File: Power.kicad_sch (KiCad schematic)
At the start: 41 parts, among them Q1 DMP2065UFDB, U6 TPS62180, U7 CYPD3177-24LQ, U8 TPS82130, U9 DS1307Z+, Y1 32.768kHz

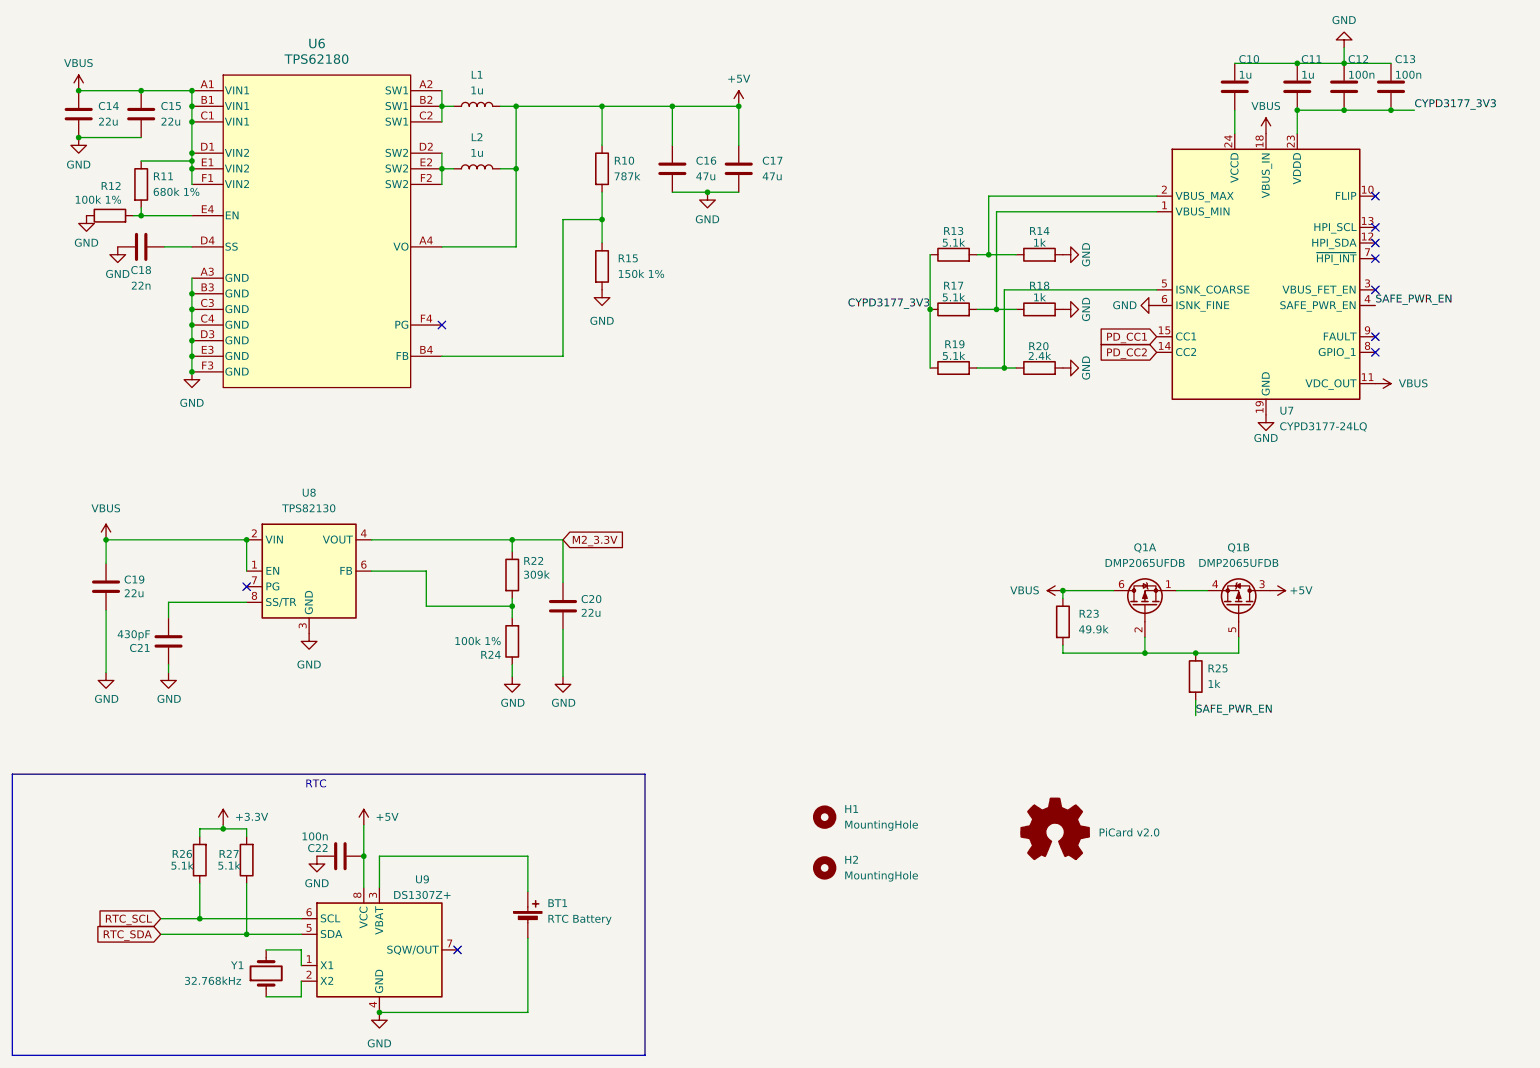
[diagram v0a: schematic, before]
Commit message: Update
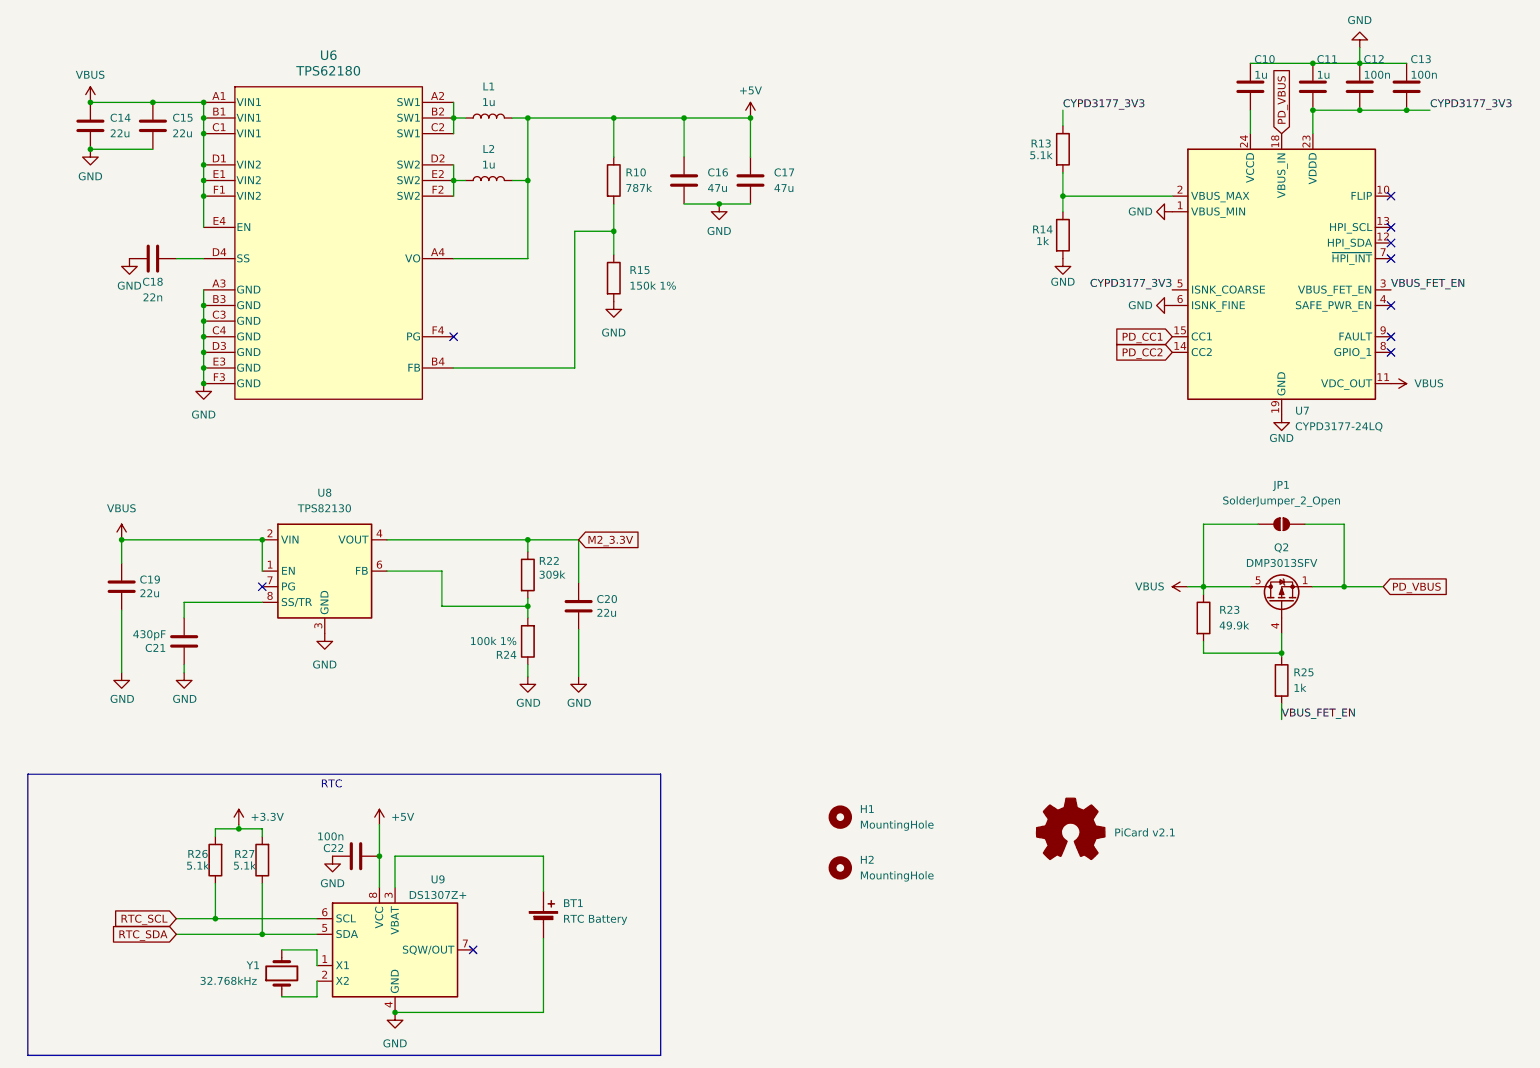
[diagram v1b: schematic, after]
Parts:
- removed Q1: DMP2065UFDB, PiCard:DFN200X200X60-8N, symbol Device:Q_Dual_PMOS_S1G1D2S2G2D1
- removed R11: 680k 1%, Resistor_SMD:R_0402_1005Metric, symbol Device:R
- removed R12: 100k 1%, Resistor_SMD:R_0402_1005Metric, symbol Device:R
- removed R17, R19: 5.1k, Resistor_SMD:R_0402_1005Metric, symbol Device:R
- removed R18: 1k, Resistor_SMD:R_0402_1005Metric, symbol Device:R
- removed R20: 2.4k, Resistor_SMD:R_0402_1005Metric, symbol Device:R
- added JP1: SolderJumper_2_Open, Jumper:SolderJumper-2_P1.3mm_Open_TrianglePad1.0x1.5mm, symbol Jumper:SolderJumper_2_Open
- added Q2: DMP3013SFV, Package_SON:Diodes_PowerDI3333-8, symbol Transistor_FET:DMP3013SFV
- SYM1: value PiCard v2.0 -> PiCard v2.1
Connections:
- net CYPD3177_3V3: now also U7.5 (ISNK_COARSE)
- net GND: now also U7.1 (VBUS_MIN)
- net VBUS: now also U6.E4 (EN), JP1.1 (A), Q2.5 (D); no longer U7.18 (VBUS_IN)
- net at R23.2, R25.1: now also Q2.4 (G)
- net VBUS_FET_EN: now reaches U7.3 (VBUS_FET_EN)
- net VBUS_FET_EN: now also R25.2
- net SAFE_PWR_EN: no longer names the net of U7.4 (SAFE_PWR_EN)
- net SAFE_PWR_EN: no longer R25.2
- new net PD_VBUS: JP1.2 (B), Q2.1 (S), Q2.2 (S), Q2.3 (S), U7.18 (VBUS_IN)
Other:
- moved on the sheet: BT1, C10, C11, C12, C13, C14, C15, C16, C17, C18, C19, C20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
